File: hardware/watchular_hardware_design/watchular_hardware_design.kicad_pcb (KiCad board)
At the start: 4 copper layers, 55.5 x 22.9 mm, 89 parts, among them J1 USB4105-GF-A, J2 665102131822, J3 TSW-116-07-H-S, J4 TSW-116-07-H-S, Q1 BSS123, Q2 BSS123, Q3 BSS123, Q4 BSS123, T1 DMG1013UW-7, U1 MCP73832T-2DCI/OT, U2 ESP32-C3FH4, U3 MIC5524-3.3YMT-TZ, U4 W25Q16JVSSIQ, U5 TL3305AF260QG, U6 TL3305AF260QG, Y1 40MHz

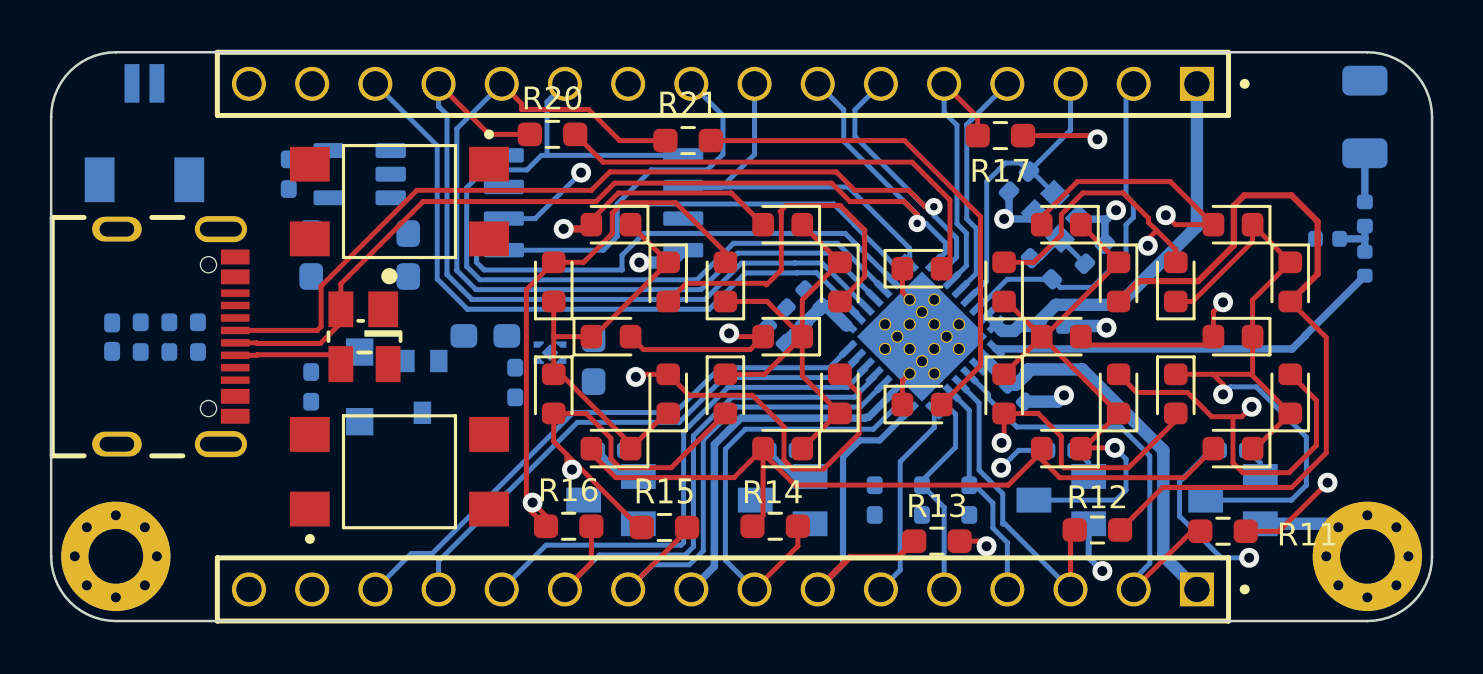
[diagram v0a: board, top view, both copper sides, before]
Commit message: Added pour zones to all the layers.
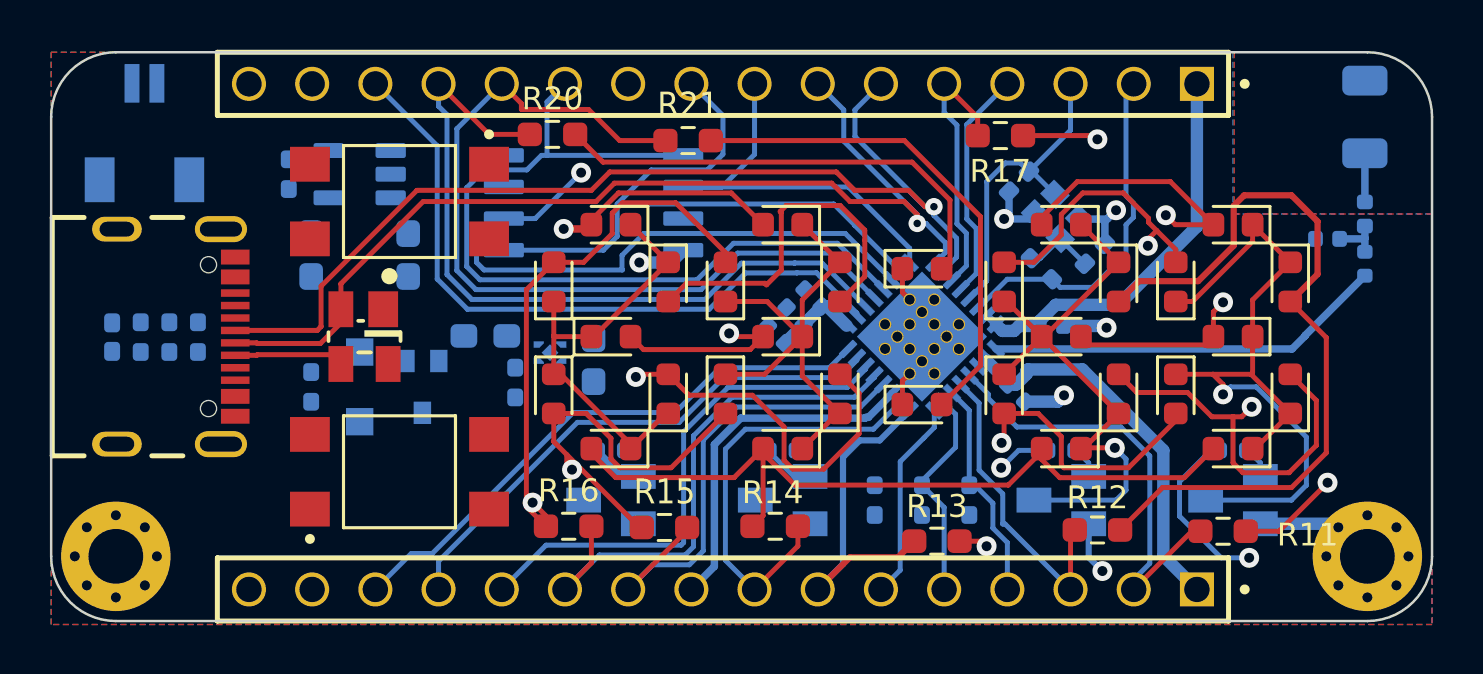
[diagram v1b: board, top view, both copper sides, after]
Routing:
- added copper zone on B.Cu, net GND
- added copper zone on F.Cu, net GND
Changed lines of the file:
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@@
   (segment (start 119.875 118.475) (end 117.742228 118.475) (width 0.2) (layer "B.Cu") (net 60))
   (segment (start 117.742228 118.475) (end 116.282228 119.935) (width 0.2) (layer "B.Cu") (net 60))
+  (zone (net 3) (net_name "GND") (layer "F.Cu") (hatch edge 0.508)
+    (connect_pads (clearance 0))
+    (min_thickness 0.25) (filled_areas_thickness no)
+    (fill yes (thermal_gap 0.5) (thermal_bridge_width 0.5))
+    (polygon
+      (pts
+        (xy 137.55 116.5)
+        (xy 145.5 116.5)
+        (xy 145.5 133)
+        (xy 90 133)
+        (xy 90 110)
+        (xy 137.55 110)
+      )
+    )
+  )
   (zone (net 43) (net_name "VDD3P3") (layer "In1.Cu") (hatch edge 0.508)
     (connect_pads (clearance 0))
@@
         (xy 90 133)
         (xy 90 110)
+        (xy 137.5 110)
+      )
+    )
+  )
+  (zone (net 3) (net_name "GND") (layer "B.Cu") (hatch edge 0.508)
+    (connect_pads (clearance 0))
+    (min_thickness 0.25) (filled_areas_thickness no)
+    (fill yes (thermal_gap 0.5) (thermal_bridge_width 0.5))
+    (polygon
+      (pts
+        (xy 137.5 116.5)
+        (xy 145.5 116.5)
+        (xy 145.5 133)
+        (xy 90 133)
+        (xy 90 110)
